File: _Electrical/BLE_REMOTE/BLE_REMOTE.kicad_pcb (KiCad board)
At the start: 4 copper layers, 49.5 x 38.5 mm, 82 parts, among them J1 PGRM, J2 Conn_01x02_Pin, J3 LED, J4 SWITCH, J5 BUZZER, J6 Display, J7 Battery, J8 USBC, Q1 BSS806NEH6327XTSA1, Q2 NPN, Q3 PMOS, SW1 SW_Push, SW2 SW_Push, SW3 SW_Push, U1 nRF52832-QFxx, U2 BQ24232RGTR, U3 MIC5528-3.3YMX-TR, U4 MCP65R41, U5 IRF7319TRPBF, Y1 Crystal_GND24

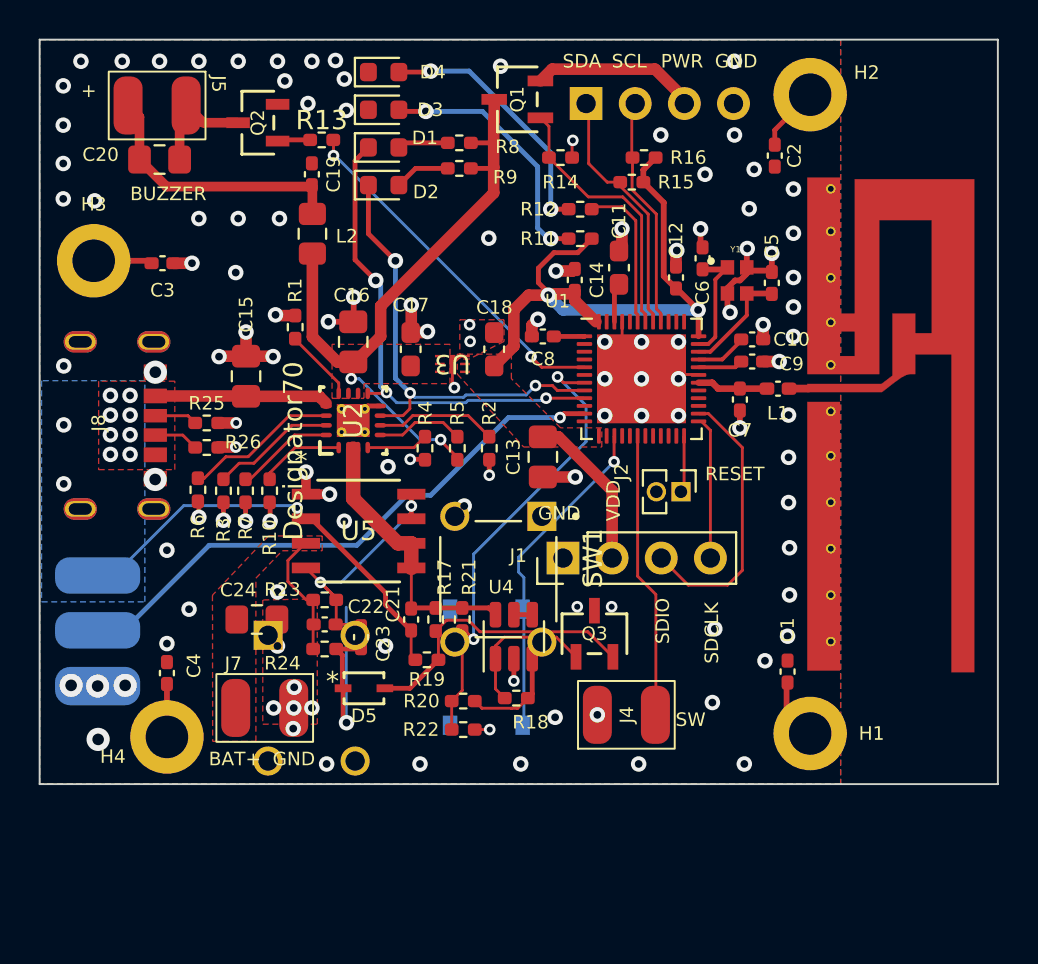
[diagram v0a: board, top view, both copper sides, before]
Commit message: asdasat
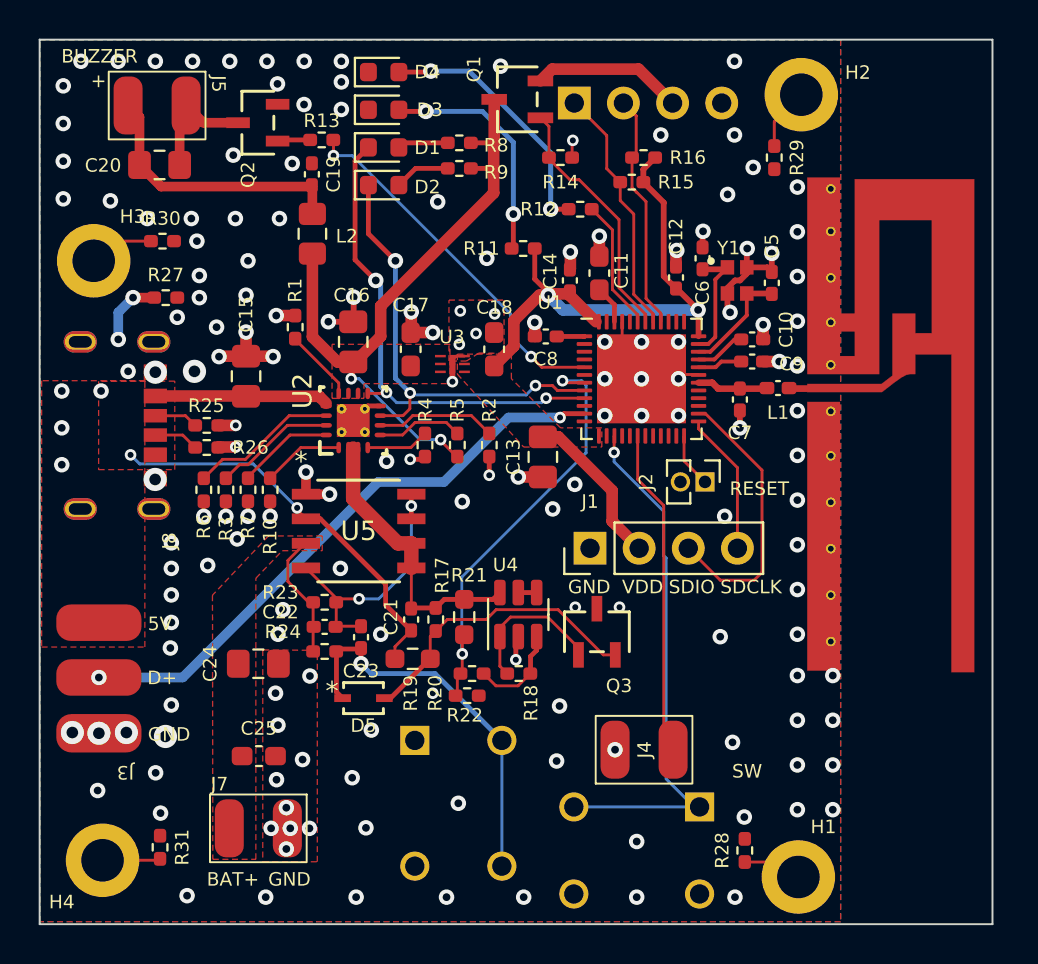
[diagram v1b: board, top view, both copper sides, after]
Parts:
- removed C1, C2, C3, C4: 0.1uF, Capacitor_SMD:C_0402_1005Metric_Pad0.74x0.62mm_HandSolder
- removed SW3: SW_Push, _Parts:SW_TS-1187A-B-A-B
- added C25: 2.2uF, Capacitor_SMD:C_0603_1608Metric_Pad1.08x0.95mm_HandSolder, F.Cu at (137.1, 117.0)
- added R27: 0R, Resistor_SMD:R_0402_1005Metric_Pad0.72x0.64mm_HandSolder, F.Cu at (132.2, 93.3)
- added R28: 0R, Resistor_SMD:R_0402_1005Metric_Pad0.72x0.64mm_HandSolder, F.Cu at (162.2, 121.9)
- added R29: 0R, Resistor_SMD:R_0402_1005Metric_Pad0.72x0.64mm_HandSolder, F.Cu at (163.7, 86.1)
- added R30: 0R, Resistor_SMD:R_0402_1005Metric_Pad0.72x0.64mm_HandSolder, F.Cu at (132.1, 90.4)
- added R31: 0R, Resistor_SMD:R_0402_1005Metric_Pad0.72x0.64mm_HandSolder, F.Cu at (132.0, 121.8)
- C22: value 0.1uF -> 100nF
- J2: value Conn_01x02_Pin -> RESET
- J3: value LED -> LED_STRIP; moved to F.Cu
- R19: footprint Resistor_SMD:R_0402_1005Metric_Pad0.72x0.64mm_HandSolder -> Resistor_SMD:R_0603_1608Metric_Pad0.98x0.95mm_HandSolder
- R21: value 178k -> 150k; footprint Resistor_SMD:R_0402_1005Metric_Pad0.72x0.64mm_HandSolder -> Resistor_SMD:R_0603_1608Metric_Pad0.98x0.95mm_HandSolder
- SW1: moved to B.Cu
- U3: value MIC5528-3.3YMX-TR -> MIC5528-3.3YMT-TR; footprint _Parts:XTDFN6_1P2X1P2_MCH -> _Parts:TDFN6_1P2X1P2_MCH
- moved SW1 15.7 mm to (156.6, 121.9), turned to 180 degrees
- moved SW2 9.33 mm to (147.4, 119.5)
- moved H1 7.44 mm to (164.9, 123.3)
- moved H4 7.19 mm to (129.0, 122.4)
- moved J7 6.23 mm to (137.0, 120.8)
- moved R11 2.99 mm to (150.7, 90.8)
- moved J3 2.44 mm to (128.8, 115.9), turned to 180 degrees
- moved C24 2.29 mm to (137.0, 112.3)
- moved J4 2.02 mm to (157.0, 116.7)
- moved R22 1.76 mm to (147.8, 113.9)
- moved R20 1.49 mm to (148.1, 112.8)
- moved J1 1.49 mm to (154.2, 106.3)
- moved J2 1.34 mm to (160.1, 102.9)
- moved R18 1.28 mm to (150.5, 112.8)
- moved U4 1.17 mm to (150.5, 109.7)
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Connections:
- J8 pad S1: GND -> SHIELD
- J8 pad S2: GND -> SHIELD
- J8 pad S3: GND -> SHIELD
- J8 pad S4: GND -> SHIELD
- SW1 pad 2: unconnected-(SW1-Pad2) -> BUTTON
- SW1 pad 3: unconnected-(SW1-Pad3) -> GND
- SW2 pad 1: unconnected-(SW2-Pad1) -> GND
- SW2 pad 4: unconnected-(SW2-Pad4) -> Net-(D5-K)
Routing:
- net BUTTON: track 17.3 -> 27.8 mm
- net Net-(D5-K): track 11.3 -> 20.1 mm
- net SHIELD: track 0.00 -> 3.57 mm, vias 0 -> 2
- net GND: track 48.2 -> 44.9 mm, vias 117 -> 166
- net VDD: track 40.9 -> 38.1 mm
- net SWITCH: track 14.8 -> 17.0 mm
- net TEST_BAT: track 24.2 -> 22.5 mm
- net +5V: track 31.4 -> 29.8 mm, vias 9 -> 2
- net Net-(D3-A): track 13.4 -> 12.1 mm
- net USER: track 7.89 -> 6.80 mm
- net LED_D: track 29.8 -> 30.7 mm, vias 1 -> 2
- net DIS_EN: track 13.8 -> 13.1 mm
- net /Peripherals/DIS_PWR: track 8.51 -> 7.81 mm
- net BUZZ: track 18.5 -> 19.0 mm
- net unconnected-(SW2-Pad4): vias 1 -> 0
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- added copper zone on In2.Cu, net SHIELD
- removed copper zone on B.Cu, net +5V
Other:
- board size 49.5 x 38.5 mm -> 49.3 x 45.7 mm
- board text added: "DODGECLOCK CONTROLLER Revision: MK5 Designer: Matthew Ebert Date 2024- MAR - 07"
- board text added: "Display"
